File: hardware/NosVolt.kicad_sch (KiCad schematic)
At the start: 41 parts, among them J101 INPUTS, J102 OUTPUTS, J103 BAT_NTC, SW101 SW_Reset, SW102 SSSS811101, U101 GMT028-05, U102 DS18B20Z, U103 ESP32-S3-WROOM-1

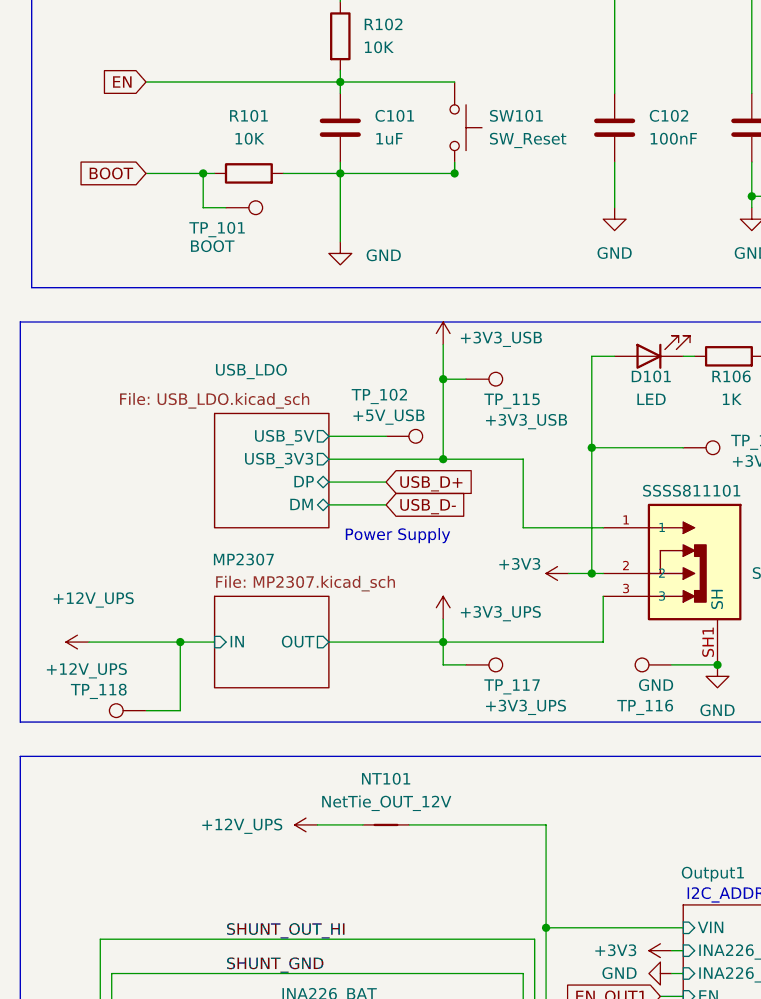
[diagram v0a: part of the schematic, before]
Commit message: PWR_FLG
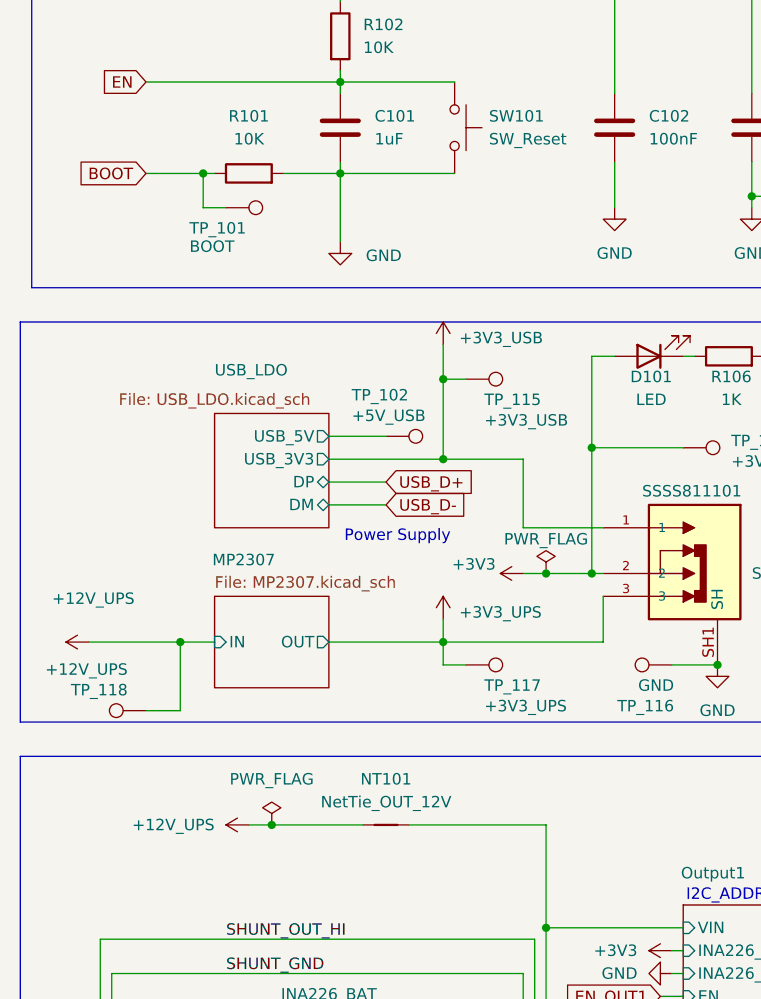
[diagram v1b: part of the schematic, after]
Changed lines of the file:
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@@
 	)
 	(junction
-		(at 69.85 45.72)
+		(at 137.16 33.02)
 		(diameter 0)
 		(color 0 0 0 0)
 	)
 	(junction
-		(at 137.16 33.02)
+		(at 49.53 118.11)
+		(diameter 0)
+		(color 0 0 0 0)
+	)
+	(junction
+		(at 80.01 90.17)
 		(diameter 0)
 		(color 0 0 0 0)
@@
 	(wire
 		(pts
-			(xy 82.55 90.17) (xy 85.09 90.17)
+			(xy 77.47 90.17) (xy 80.01 90.17)
 		)
 		(stroke
@@
 	(wire
 		(pts
-			(xy 54.61 118.11) (xy 59.69 118.11)
+			(xy 49.53 118.11) (xy 59.69 118.11)
+		)
+		(stroke
+			(width 0)
+			(type default)
+		)
+	)
+	(wire
+		(pts
+			(xy 46.99 118.11) (xy 49.53 118.11)
 		)
 		(stroke
@@
 	(wire
 		(pts
-			(xy 69.85 44.45) (xy 69.85 45.72)
+			(xy 80.01 90.17) (xy 85.09 90.17)
 		)
 		(stroke
@@
 	(symbol
 		(lib_id "power:+3.3V")
-		(at 82.55 90.17 90)
+		(at 77.47 90.17 90)
 		(unit 1)
 		(exclude_from_sim no)
@@
 		(dnp no)
 		(property "Reference" "#PWR0111"
-			(at 86.36 90.17 0)
+			(at 81.28 90.17 0)
 			(effects
 				(font
@@
 		)
 		(property "Value" "+3V3"
-			(at 79.502 89.154 90)
+			(at 74.422 89.154 90)
 			(effects
 				(font
@@
 		)
 		(property "Footprint" ""
-			(at 82.55 90.17 0)
+			(at 77.47 90.17 0)
 			(effects
 				(font
@@
 		)
 		(property "Datasheet" ""
-			(at 82.55 90.17 0)
+			(at 77.47 90.17 0)
 			(effects
 				(font
@@
 		)
 		(property "Description" "Power symbol creates a global label with name \"+3.3V\""
-			(at 82.55 90.17 0)
+			(at 77.47 90.17 0)
 			(effects
 				(font
@@
 	)
 	(symbol
+		(lib_id "power:PWR_FLAG")
+		(at 49.53 118.11 0)
+		(unit 1)
+		(exclude_from_sim no)
+		(in_bom yes)
+		(on_board yes)
+		(dnp no)
+		(fields_autoplaced yes)
+		(property "Reference" "#FLG0101"
+			(at 49.53 116.205 0)
+			(effects
+				(font
+					(size 1.27 1.27)
+				)
+				(hide yes)
+			)
+		)
+		(property "Value" "PWR_FLAG"
+			(at 49.53 113.03 0)
+			(effects
+				(font
+					(size 1.27 1.27)
+				)
+			)
+		)
+		(property "Footprint" ""
+			(at 49.53 118.11 0)
+			(effects
+				(font
+					(size 1.27 1.27)
+				)
+				(hide yes)
+			)
+		)
+		(property "Datasheet" "~"
+			(at 49.53 118.11 0)
+			(effects
+				(font
+					(size 1.27 1.27)
+				)
+				(hide yes)
+			)
+		)
+		(property "Description" "Special symbol for telling ERC where power comes from"
+			(at 49.53 118.11 0)
+			(effects
+				(font
+					(size 1.27 1.27)
+				)
+				(hide yes)
+			)
+		)
+		(pin "1"
+		)
+		(instances
+			(project "NosVolt"
+				(path "/2a3ef4c2-927a-45cd-a4f2-5ee83a7e9444"
+					(reference "#FLG0101")
+					(unit 1)
+				)
+			)
+		)
+	)
+	(symbol
 		(lib_id "Mechanical:MountingHole_Pad")
 		(at 265.43 144.78 0)
@@
 	(symbol
 		(lib_id "power:+12V")
-		(at 54.61 118.11 90)
+		(at 46.99 118.11 90)
 		(unit 1)
 		(exclude_from_sim no)
@@
 		(fields_autoplaced yes)
 		(property "Reference" "#PWR0106"
-			(at 58.42 118.11 0)
+			(at 50.8 118.11 0)
 			(effects
 				(font
@@
 		)
 		(property "Value" "+12V_UPS"
-			(at 50.8 118.1099 90)
+			(at 43.18 118.1099 90)
 			(effects
 				(font
@@
 		)
 		(property "Footprint" ""
-			(at 54.61 118.11 0)
+			(at 46.99 118.11 0)
 			(effects
 				(font
@@
 		)
 		(property "Datasheet" ""
-			(at 54.61 118.11 0)
+			(at 46.99 118.11 0)
 			(effects
 				(font
@@
 		)
 		(property "Description" "Power symbol creates a global label with name \"+12V\""
-			(at 54.61 118.11 0)
+			(at 46.99 118.11 0)
 			(effects
 				(font
@@
 					(unit 1)
 				)
+			)
+		)
+	)
+	(symbol
+		(lib_id "power:PWR_FLAG")
+		(at 80.01 90.17 0)
+		(unit 1)
+		(exclude_from_sim no)
+		(in_bom yes)
+		(on_board yes)
+		(dnp no)
+		(property "Reference" "#FLG0102"
+			(at 80.01 88.265 0)
+			(effects
+				(font
+					(size 1.27 1.27)
+				)
+				(hide yes)
+			)
+		)
+		(property "Value" "PWR_FLAG"
+			(at 80.01 86.36 0)
+			(effects
+				(font
+					(size 1.27 1.27)
+				)
+			)
+		)
+		(property "Footprint" ""
+			(at 80.01 90.17 0)
+			(effects
+				(font
+					(size 1.27 1.27)
+				)
+				(hide yes)
+			)
+		)
+		(property "Datasheet" "~"
+			(at 80.01 90.17 0)
+			(effects
+				(font
+					(size 1.27 1.27)
+				)
+				(hide yes)
+			)
+		)
+		(property "Description" "Special symbol for telling ERC where power comes from"
+			(at 80.01 90.17 0)
+			(effects
+				(font
+					(size 1.27 1.27)
+				)
+				(hide yes)
+			)
+		)
+		(pin "1"
+		)
+		(instances
+			(project "NosVolt"
+				(path "/2a3ef4c2-927a-45cd-a4f2-5ee83a7e9444"
+					(reference "#FLG0102")
+					(unit 1)
+				)
